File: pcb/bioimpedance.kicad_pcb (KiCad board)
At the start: 2 copper layers, 42.5 x 70 mm, 44 parts, among them J1 Conn_01x05_Pin, J3 USB_C_Receptacle_USB2.0_16P, J6 Conn_01x16_Pin, J8 Conn_01x16_Pin, SW5 SW_Push, SW6 SW_Push, U1 ESP32-S3-WROOM-1, U2 MAX30001CWV_T, U3 AP2112K-3.3, U4 AP2112K-1.8, Y1 OK322532.768KJBA4SL

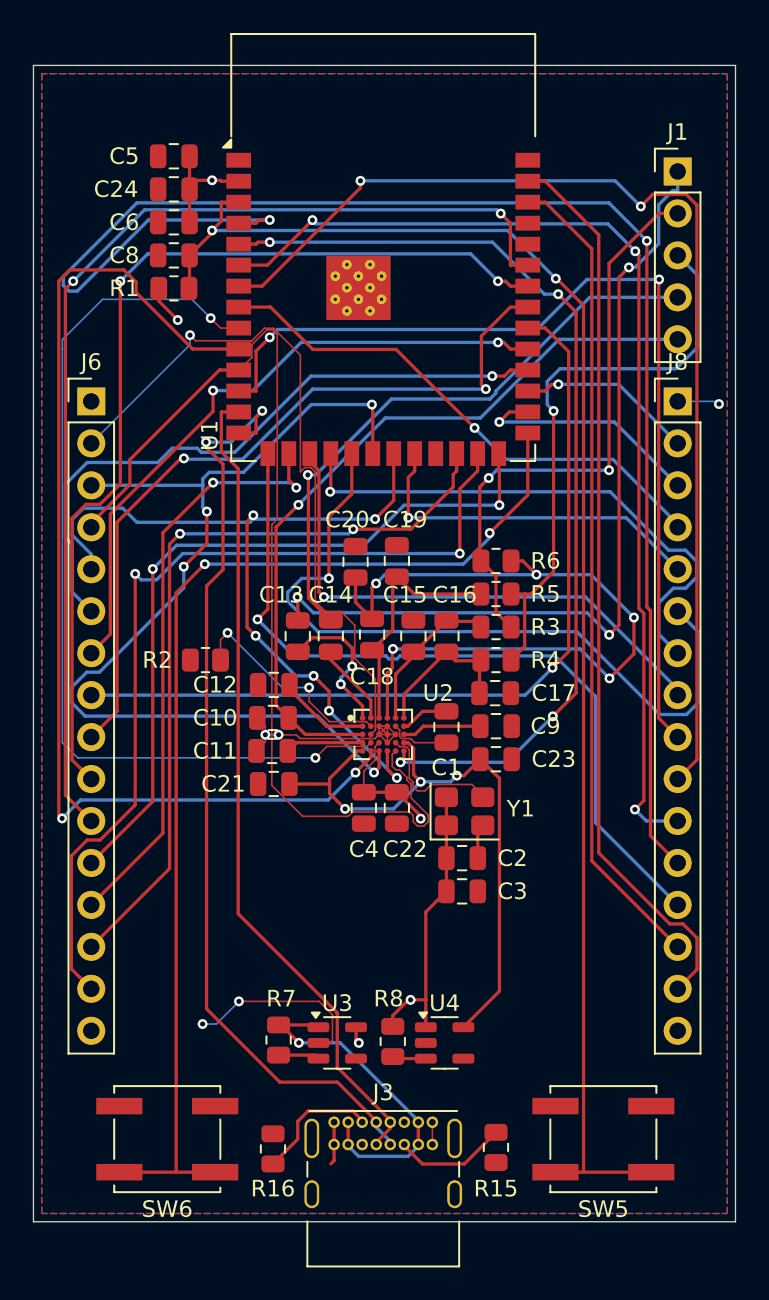
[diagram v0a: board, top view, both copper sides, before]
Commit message: reroute pcb
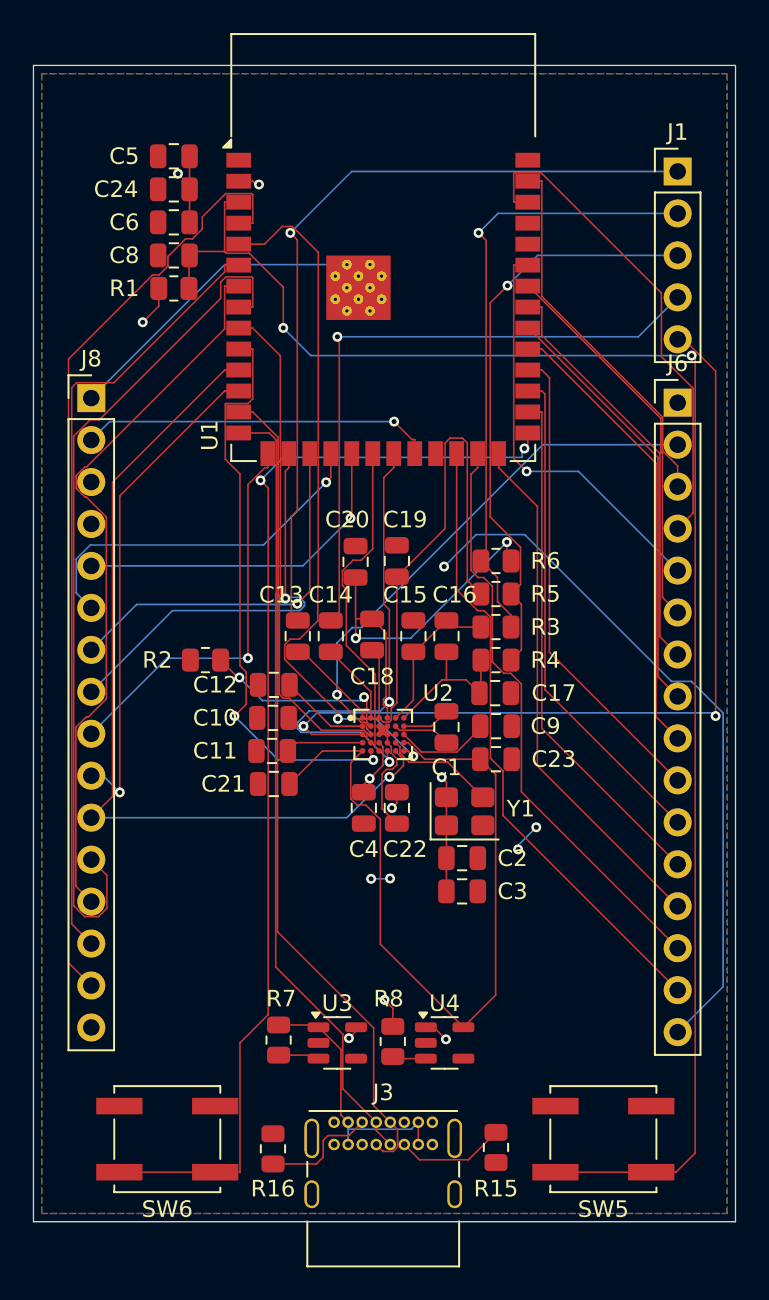
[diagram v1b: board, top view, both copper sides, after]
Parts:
- moved J8 35.5 mm to (96.0, 50.1)
- moved J6 35.5 mm to (131.5, 50.4)
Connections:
- J6 pad 10: 41 -> 37
- J6 pad 11: 42 -> 36
- J6 pad 12: 45 -> 35
- J6 pad 13: 46 -> 45
- J6 pad 14: 47 -> 48
- J6 pad 15: 48 -> 47
- J6 pad 3: MISO -> 01
- J6 pad 4: SCLK -> 02
- J6 pad 5: MOSI -> 42
- J6 pad 6: 37 -> 41
- J6 pad 7: 38 -> 40
- J6 pad 9: 40 -> 38
- J8 pad 10: 07 -> 08
- J8 pad 11: 06 -> SCLK
- J8 pad 12: 04 -> 15
- J8 pad 13: 03 -> 07
- J8 pad 14: 02 -> 06
- J8 pad 15: 01 -> 04
- J8 pad 2: 36 -> 14
- J8 pad 3: 35 -> 13
- J8 pad 4: 15 -> 12
- J8 pad 5: 14 -> 11
- J8 pad 6: 11 -> 10
- J8 pad 7: 10 -> 09
- J8 pad 8: 09 -> 46
- J8 pad 9: 08 -> 03
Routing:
- net GND: track 36.0 -> 77.2 mm
- net MISO: track 60.8 -> 20.0 mm, vias 4 -> 0
- net 42: track 65.7 -> 25.3 mm, vias 2 -> 1
- net 04: track 93.5 -> 57.2 mm, vias 2 -> 0
- net 41: track 58.5 -> 23.5 mm, vias 2 -> 0
- net 01: track 54.7 -> 22.7 mm
- net INT2B: track 66.7 -> 35.5 mm
- net 08: track 57.9 -> 29.9 mm, vias 2 -> 1
- net INTB: track 56.3 -> 30.7 mm, vias 2 -> 0
- net 39: track 51.2 -> 26.1 mm, vias 1 -> 0
- net 11: track 45.5 -> 20.8 mm
- net 07: track 67.1 -> 43.9 mm, vias 2 -> 0
- net 03: track 47.5 -> 24.4 mm
- net Net-(U2-BIP): track 46.4 -> 24.0 mm, vias 5 -> 2
- net 40: track 46.2 -> 25.3 mm, vias 2 -> 0
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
